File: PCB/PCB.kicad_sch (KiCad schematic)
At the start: 32 parts, among them SW1 SW_Push, SW10 SW_Push, SW11 SW_Push, SW12 SW_Push, SW13 RotaryEncoder_Switch, SW2 SW_Push, SW3 SW_Push, SW4 SW_Push, SW5 SW_Push, SW6 SW_Push, SW7 SW_Push, SW8 SW_Push, SW9 SW_Push, U1 MOUDLE-SEEEDUINO-XIAO

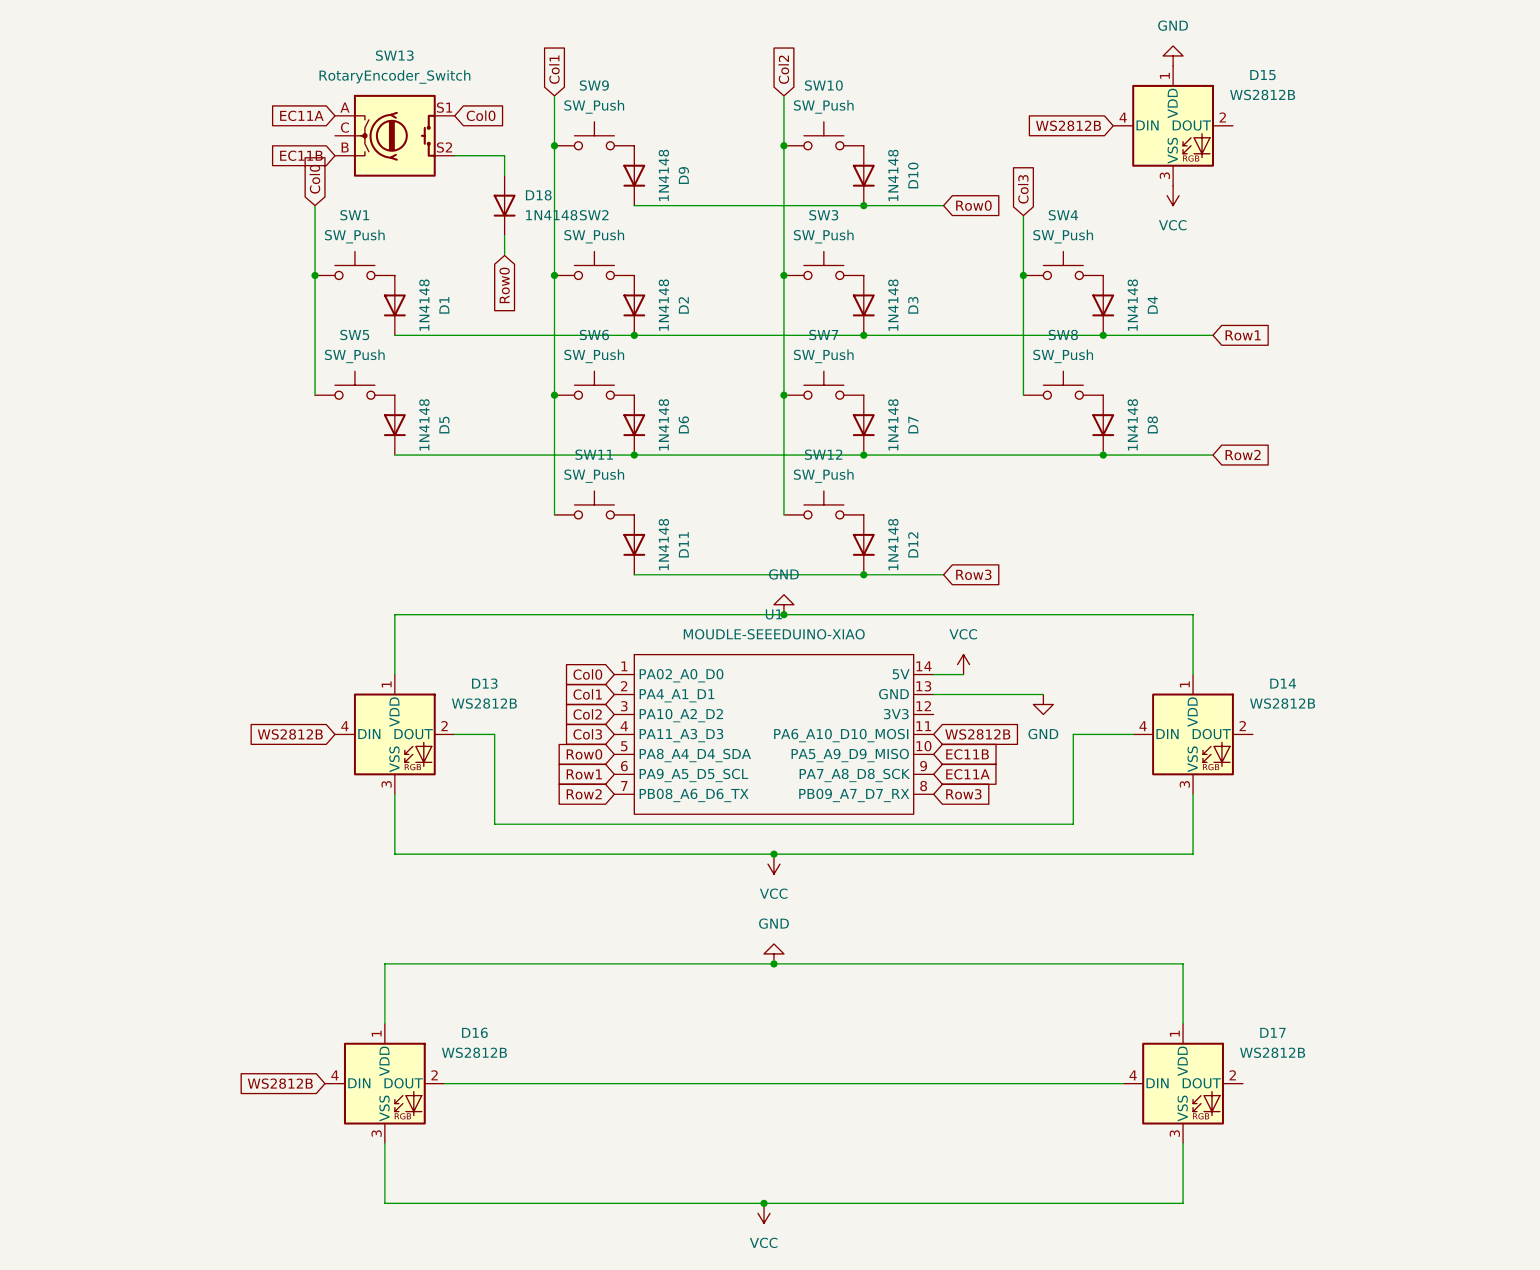
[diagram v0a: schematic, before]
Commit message: Add files via upload
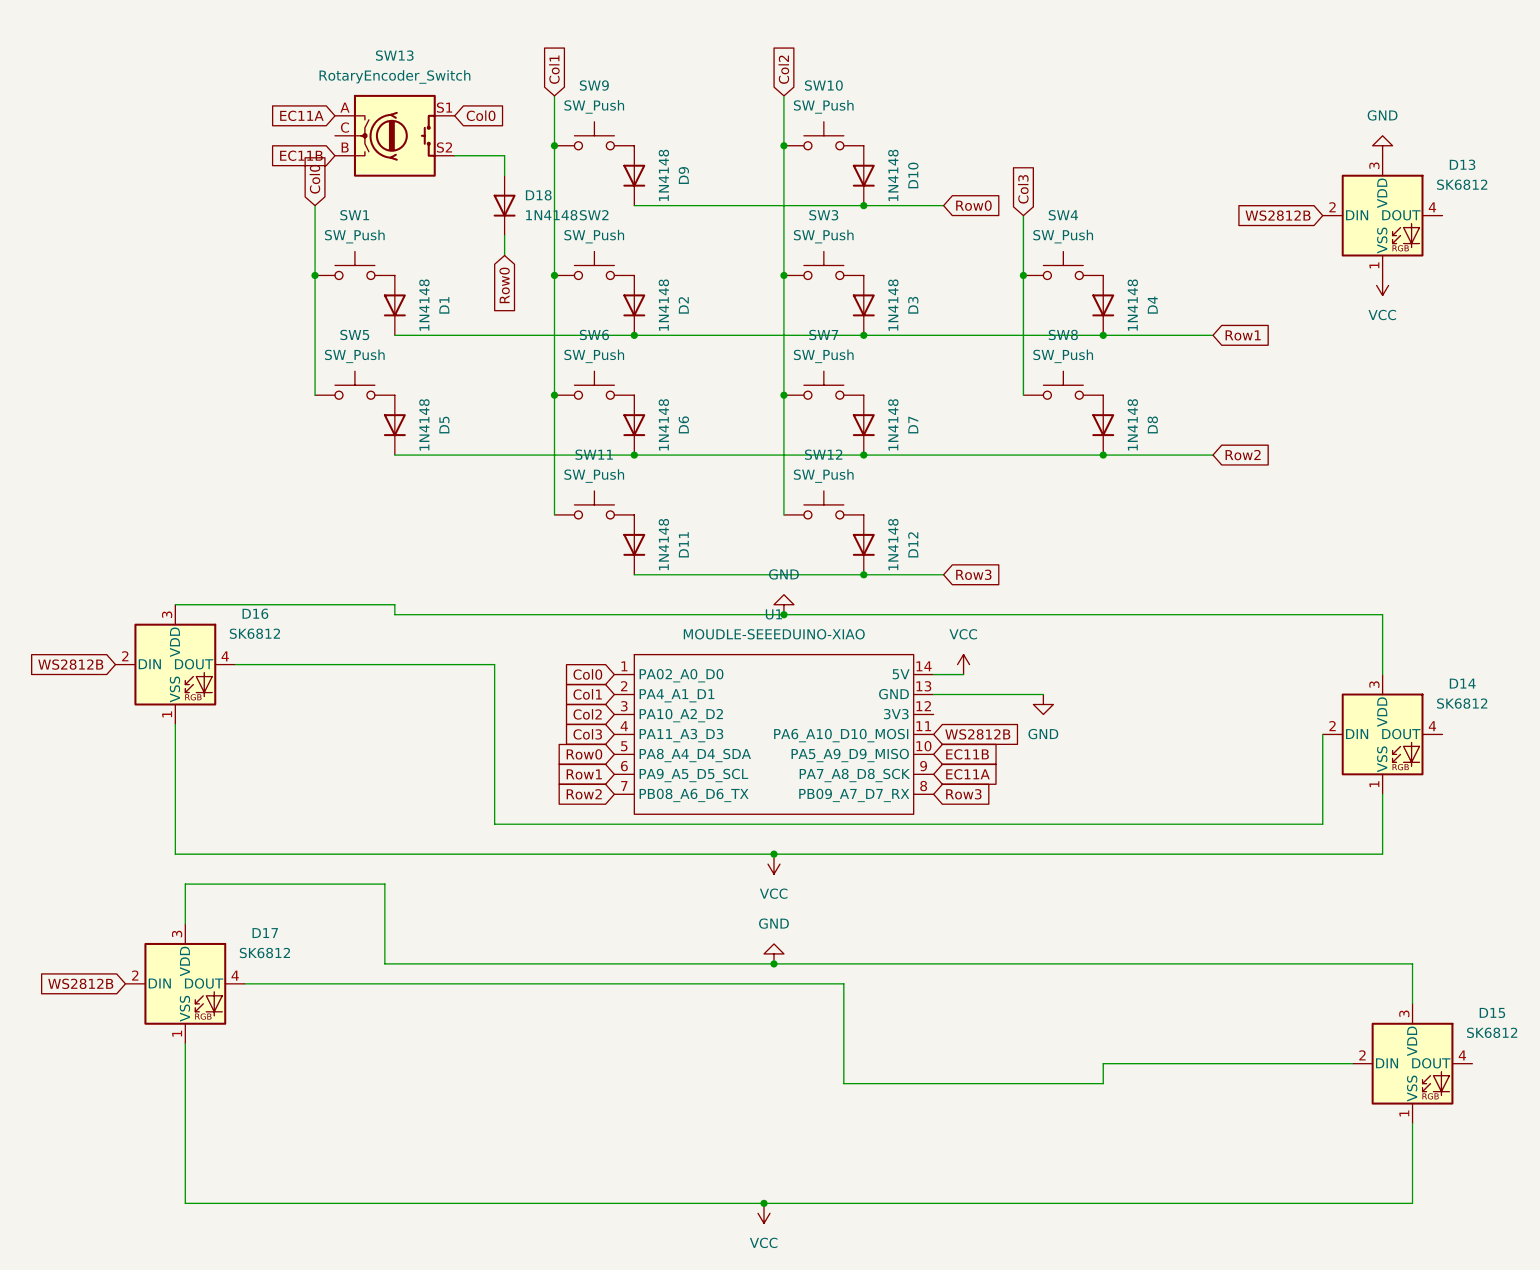
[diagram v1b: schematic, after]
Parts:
- removed D13, D14, D15, D16, D17: WS2812B, LED_SMD:LED_WS2812B_PLCC4_5.0x5.0mm_P3.2mm, symbol LED:WS2812B
- added D13, D14, D15, D16, D17: SK6812, LED_SMD:LED_SK6812_PLCC4_5.0x5.0mm_P3.2mm, symbol LED:SK6812
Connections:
- net GND: now also D13.3 (VDD), D14.3 (VDD), D15.3 (VDD), D16.3 (VDD), D17.3 (VDD)
- net VCC: now also D13.1 (VSS), D14.1 (VSS), D15.1 (VSS), D16.1 (VSS), D17.1 (VSS)
- net WS2812B: now also D13.2 (DIN), D16.2 (DIN), D17.2 (DIN)
- new net: D15.2 (DIN), D17.4 (DOUT)
- new net: D14.2 (DIN), D16.4 (DOUT)
